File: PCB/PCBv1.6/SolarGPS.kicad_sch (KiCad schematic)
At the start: 44 parts, among them J1 Conn_01x10_Female, J2 Solar2+, J3 Solar1+, J4 GND, J5 GND, J6 Conn_02x03_Odd_Even, J7 Screw_Terminal_01x01, J8 Conn_01x04_Male, U1 BQ25505, U2 L96-M33, U3 STM32L031G6Ux, U4 MAX40200AUK, U6 LIS3DH, Y1 32.768

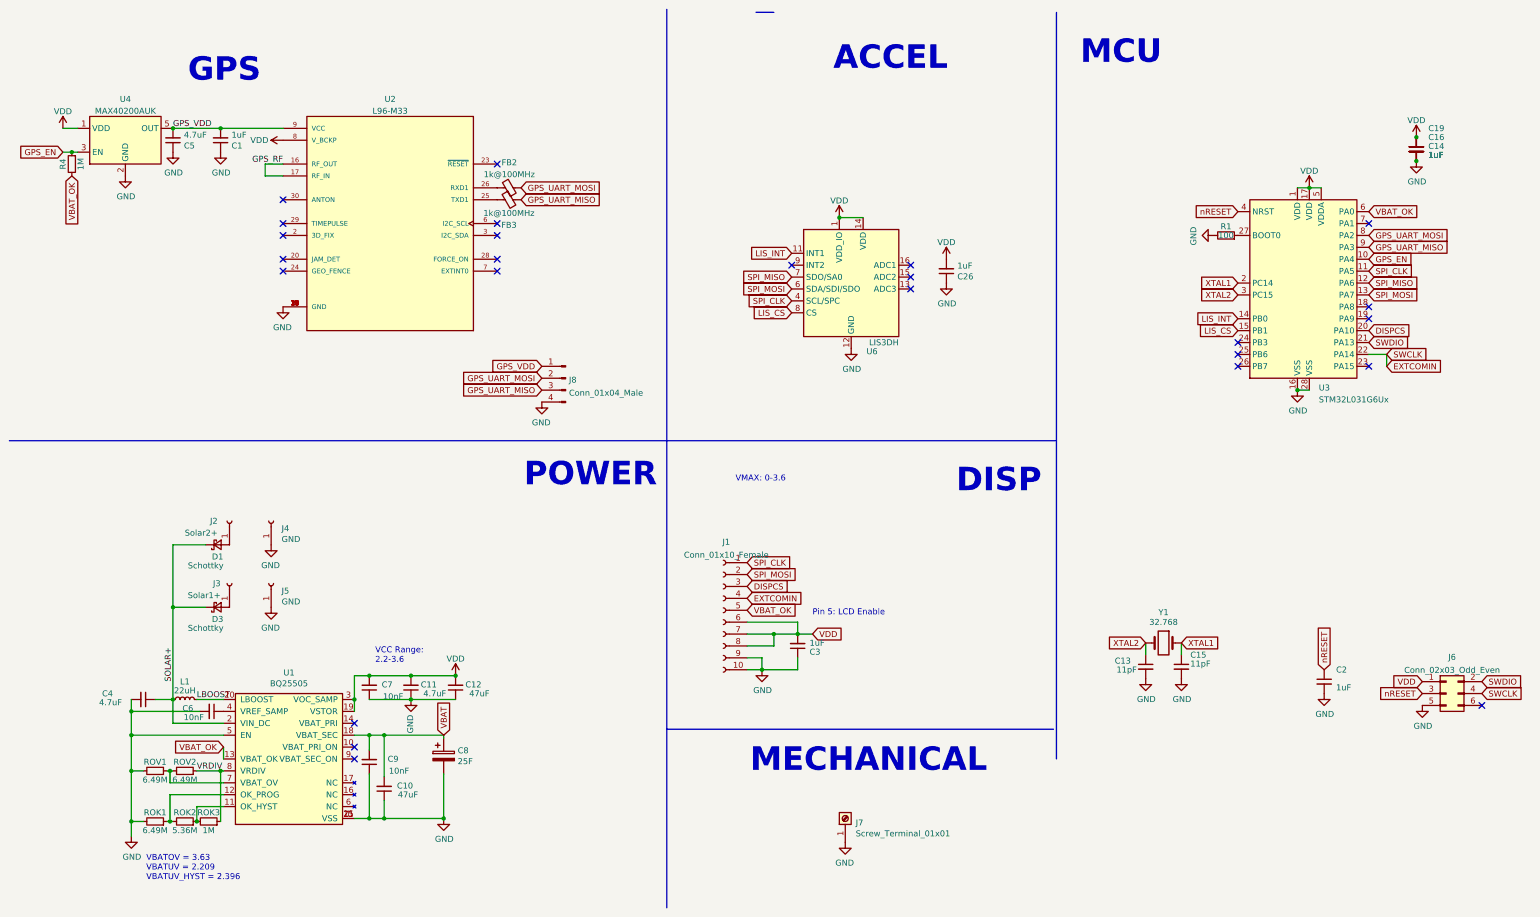
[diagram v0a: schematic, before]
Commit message: Update PCBV10
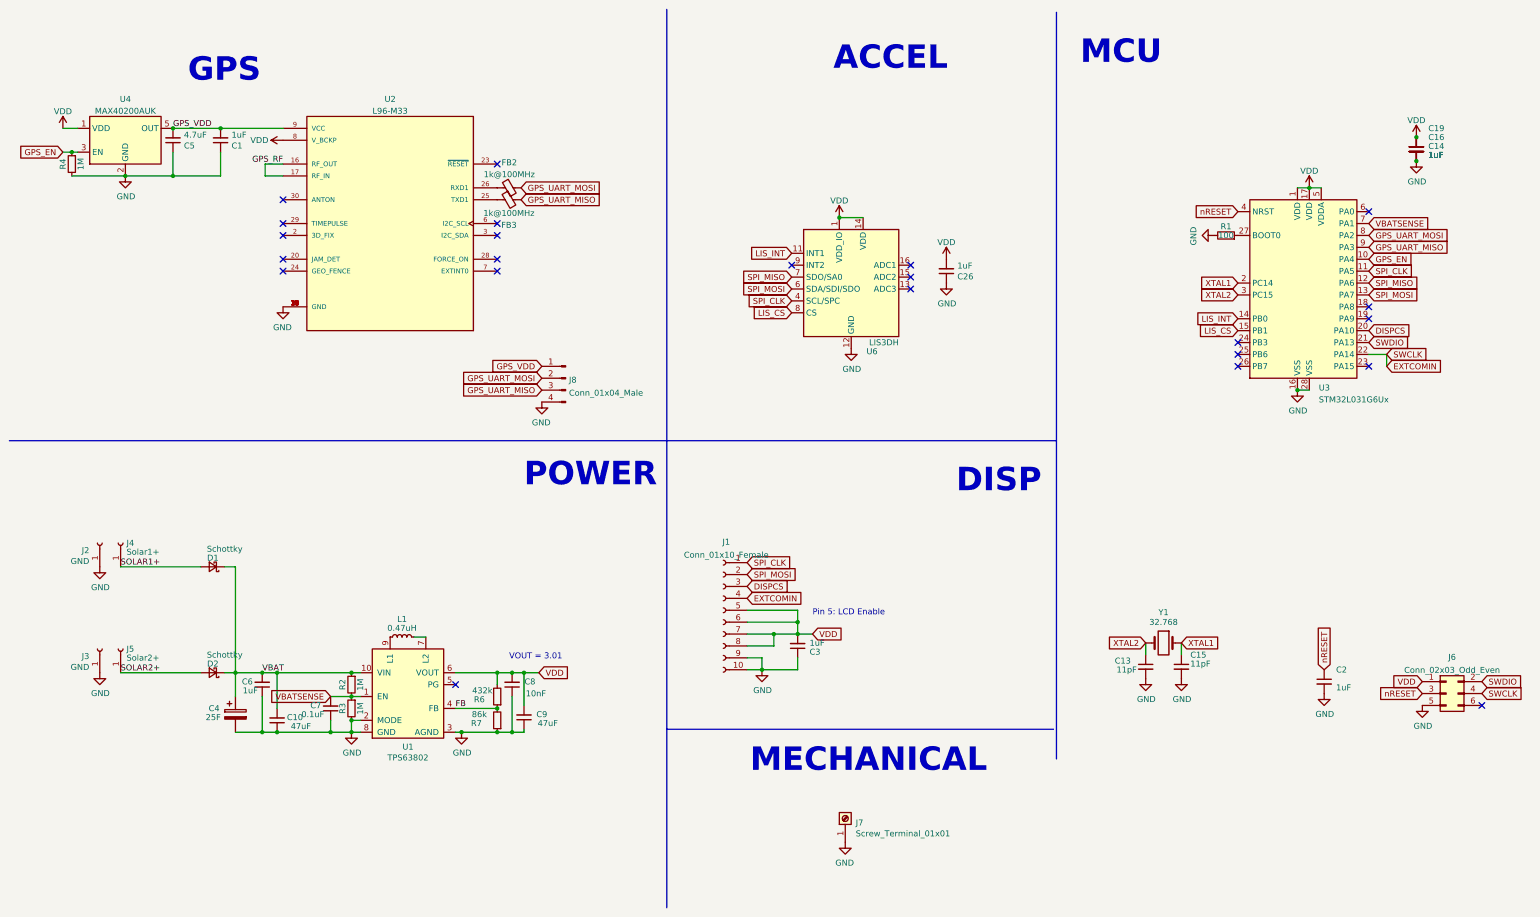
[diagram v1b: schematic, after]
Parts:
- removed C11, C4: 4.7uF, Capacitor_SMD:C_0805_2012Metric, symbol Device:C_Small
- removed C12: 47uF, Capacitor_SMD:C_1206_3216Metric, symbol Device:C_Small
- removed C8: 25F, Heliograph:TPLC3R8-25MR8X20, symbol Device:C_Polarized
- removed D3: Schottky, Diode_SMD:D_SOD-323_HandSoldering, symbol Device:D_Schottky_Small
- removed ROK1, ROV1, ROV2: 6.49M, Resistor_SMD:R_0603_1608Metric, symbol Device:R_Small
- removed ROK2: 5.36M, Resistor_SMD:R_0603_1608Metric, symbol Device:R_Small
- removed ROK3: 1M, Resistor_SMD:R_0603_1608Metric, symbol Device:R_Small
- removed U1: BQ25505, Package_DFN_QFN:Texas_VQFN-RGR-20, symbol MargoGeneral:BQ25505
- added C4: 25F, Heliograph:TPLC3R8-25MR8X20, symbol Device:C_Polarized
- added C8: 10nF, Capacitor_SMD:C_0603_1608Metric, symbol Device:C_Small
- added D2: Schottky, Diode_SMD:D_SOD-323_HandSoldering, symbol Device:D_Schottky_Small
- added R2, R3: 1M, Resistor_SMD:R_0603_1608Metric, symbol Device:R_Small
- added R6: 432k, Resistor_SMD:R_0603_1608Metric, symbol Device:R_Small
- added R7: 86k, Resistor_SMD:R_0603_1608Metric, symbol Device:R_Small
- added U1: TPS63802, Margo_Lib:VREG_TPS63802DLAR, symbol SolarGPS-rescue:TPS63802-VeridianDesigns
- C6: value 10nF -> 1uF
- C7: value 10nF -> 0.1uF
- C9: value 10nF -> 47uF; footprint Capacitor_SMD:C_0603_1608Metric -> Capacitor_SMD:C_1206_3216Metric
- J2: value Solar2+ -> GND
- J3: value Solar1+ -> GND
- J4: value GND -> Solar1+
- J5: value GND -> Solar2+
- L1: value 22uH -> 0.47uH; footprint Heliograph:744031220 -> Inductor_SMD:L_0805_2012Metric_Pad1.05x1.20mm_HandSolder; Part 744031220 -> DFE201612E
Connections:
- net GND: now also C6.1, J2.1 (Pin_1), J3.1 (Pin_1), R4.2, C4.2, C8.1, R3.2, R7.1, U1.2 (MODE), U1.3 (AGND), U1.8 (GND); no longer C6.2, J4.1 (Pin_1), J5.1 (Pin_1)
- net VBAT: now also C6.2, D1.1 (K), C4.1, D2.1 (K), R2.1, U1.10 (VIN); no longer C9.2
- net VDD: now also C9.2, J1.5 (Pin_5), C8.2, R6.2, U1.6 (VOUT); no longer C7.2
- net VBATSENSE: now reaches U3.7 (PA1)
- net VBATSENSE: now also C7.2, R2.2, R3.1, U1.1 (EN)
- net SOLAR1+: now reaches D1.2 (A)
- net SOLAR1+: now also J4.1 (Pin_1); no longer J2.1 (Pin_1)
- net LBOOST: no longer names the net of L1.2
- net LBOOST: now also U1.7 (L2)
- net SOLAR+: no longer names the net of L1.1
- net SOLAR+: now also U1.9 (L1); no longer D1.1 (K)
- removed net VBAT_OK: J1.5 (Pin_5), R4.2, U3.6 (PA0)
- new net FB: R6.1, R7.2, U1.4 (FB)
- new net SOLAR2+: D2.2 (A), J5.1 (Pin_1)
- no-connect marks 25 -> 23
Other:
- note added: "VOUT = 3.01"
- note removed: "VBATOV = 3.63 VBATUV = 2.209 VBATUV_HYST = 2.396"
- note removed: "VCC Range: 2.2-3.6"
- note removed: "VMAX: 0-3.6"

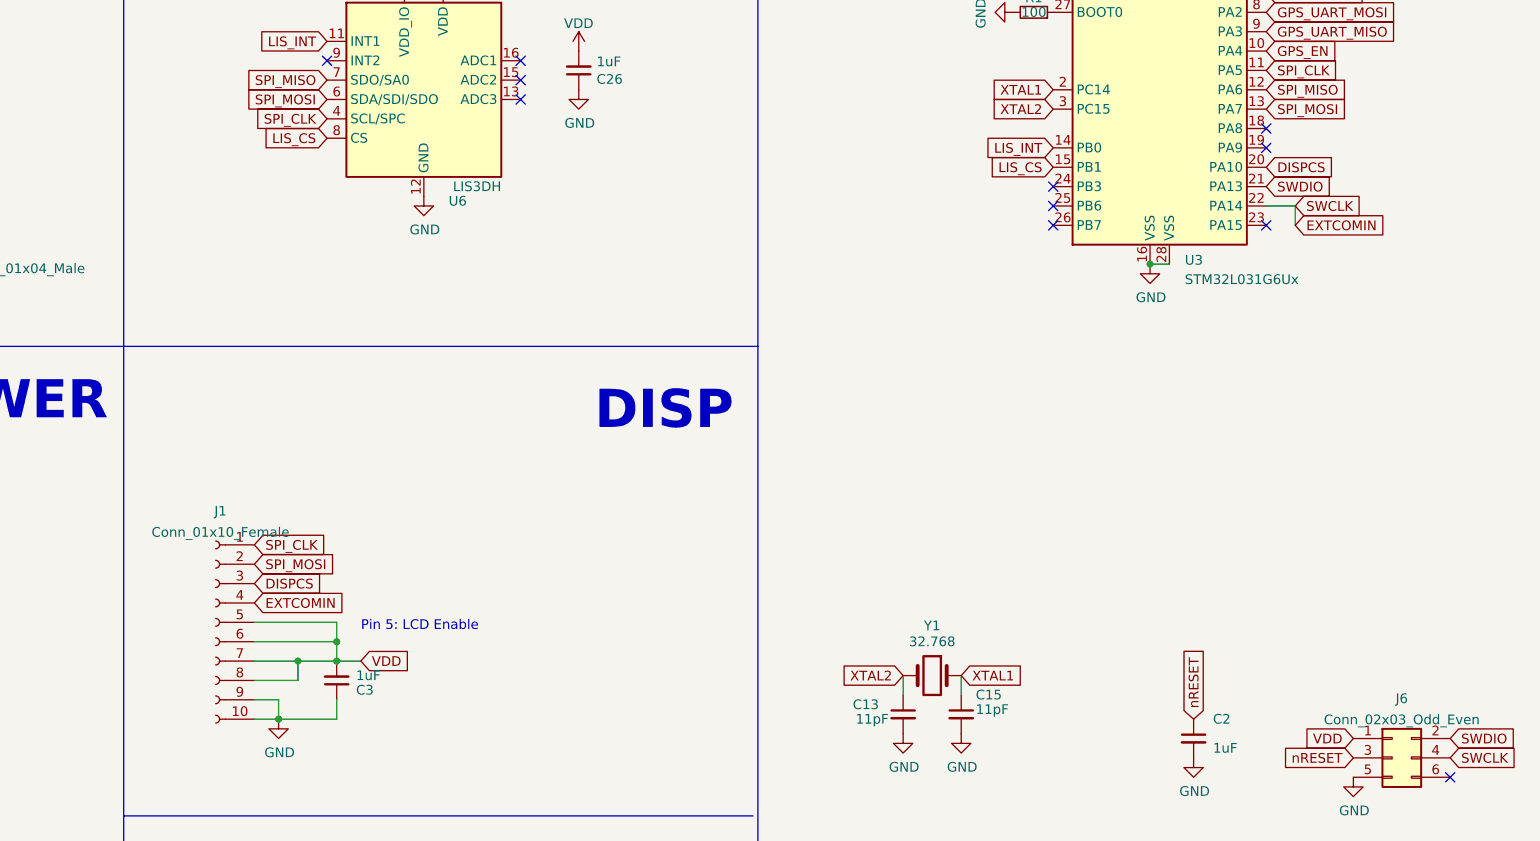
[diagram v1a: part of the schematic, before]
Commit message: PCB1.6
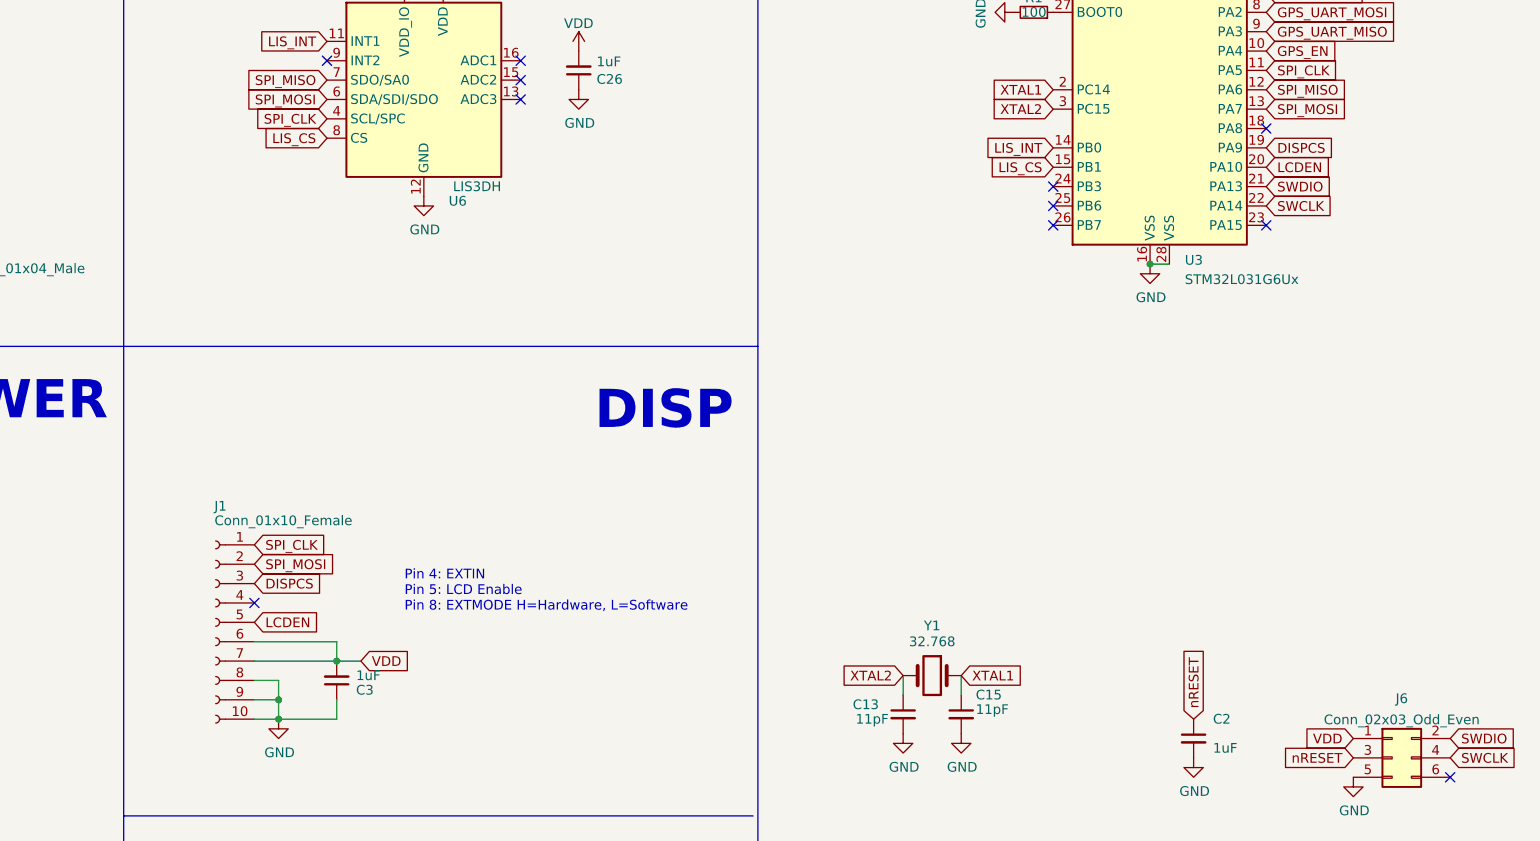
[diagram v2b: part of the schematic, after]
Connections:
- net DISPCS: now also U3.19 (PA9); no longer U3.20 (PA10)
- net GND: now also J1.8 (Pin_8)
- net VDD: no longer J1.5 (Pin_5), J1.8 (Pin_8)
- net EXTCOMIN renamed SWCLK
- net SWCLK: no longer J1.4 (Pin_4)
- new net LCDEN: J1.5 (Pin_5), U3.20 (PA10)
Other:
- note added: "Pin 4: EXTIN Pin 5: LCD Enable Pin 8: EXTMODE H=Hardware, L=Software"
- note removed: "Pin 5: LCD Enable"
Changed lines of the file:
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@@
   (junction (at 66.04 153.035) (diameter 0) (color 0 0 0 0)
   )
-  (junction (at 180.34 142.24) (diameter 0) (color 0 0 0 0)
-  )
   (junction (at 57.15 36.83) (diameter 0) (color 0 0 0 0)
   )
@@
   (junction (at 85.09 163.195) (diameter 0) (color 0 0 0 0)
   )
+  (junction (at 172.72 149.86) (diameter 0) (color 0 0 0 0)
+  )
   (junction (at 66.04 165.735) (diameter 0) (color 0 0 0 0)
   )
@@
   (junction (at 119.38 165.735) (diameter 0) (color 0 0 0 0)
   )
-  (junction (at 175.26 144.78) (diameter 0) (color 0 0 0 0)
-  )
   (junction (at 46.99 46.99) (diameter 0) (color 0 0 0 0)
   )
-  (no_connect (at 302.26 77.47))
+  (no_connect (at 169.545 137.16))
   (no_connect (at 204.47 71.12))
   (no_connect (at 107.315 155.575))
@@
     (stroke (width 0) (type default) (color 0 0 0 0))
   )
-  (wire (pts (xy 180.34 139.7) (xy 169.545 139.7))
-    (stroke (width 0) (type default) (color 0 0 0 0))
-  )
   (wire (pts (xy 172.72 149.86) (xy 172.72 152.4))
     (stroke (width 0) (type default) (color 0 0 0 0))
@@
     (stroke (width 0) (type default) (color 0 0 0 0))
   )
-  (wire (pts (xy 175.26 147.32) (xy 175.26 144.78))
+  (wire (pts (xy 172.72 149.86) (xy 172.72 147.32))
     (stroke (width 0) (type default) (color 0 0 0 0))
   )
@@
     (stroke (width 0) (type default) (color 0 0 0 0))
   )
+  (wire (pts (xy 172.72 147.32) (xy 169.545 147.32))
+    (stroke (width 0) (type default) (color 0 0 0 0))
+  )
   (polyline (pts (xy 12.065 103.505) (xy 235.585 103.505))
     (stroke (width 0) (type default) (color 0 0 0 0))
@@
     (stroke (width 0) (type default) (color 0 0 0 0))
   )
-  (wire (pts (xy 169.545 147.32) (xy 175.26 147.32))
-    (stroke (width 0) (type default) (color 0 0 0 0))
-  )
   (wire (pts (xy 85.09 163.195) (xy 86.995 163.195))
     (stroke (width 0) (type default) (color 0 0 0 0))
@@
     (stroke (width 0) (type default) (color 0 0 0 0))
   )
-  (wire (pts (xy 169.545 144.78) (xy 175.26 144.78))
+  (wire (pts (xy 169.545 144.78) (xy 180.34 144.78))
     (stroke (width 0) (type default) (color 0 0 0 0))
   )
@@
     (stroke (width 0) (type default) (color 0 0 0 0))
   )
-  (wire (pts (xy 180.34 142.24) (xy 180.34 139.7))
-    (stroke (width 0) (type default) (color 0 0 0 0))
-  )
   (wire (pts (xy 25.4 46.99) (xy 36.83 46.99))
     (stroke (width 0) (type default) (color 0 0 0 0))
   )
-  (wire (pts (xy 175.26 144.78) (xy 180.34 144.78))
-    (stroke (width 0) (type default) (color 0 0 0 0))
-  )
   (wire (pts (xy 85.09 163.195) (xy 85.09 165.735))
     (stroke (width 0) (type default) (color 0 0 0 0))
@@
     (stroke (width 0) (type default) (color 0 0 0 0))
   )
-  (wire (pts (xy 302.26 85.09) (xy 306.07 85.09))
-    (stroke (width 0) (type default) (color 0 0 0 0))
-  )
   (wire (pts (xy 36.83 46.99) (xy 46.99 46.99))
     (stroke (width 0) (type default) (color 0 0 0 0))
@@
   )
   (wire (pts (xy 107.315 153.035) (xy 116.205 153.035))
-    (stroke (width 0) (type default) (color 0 0 0 0))
-  )
-  (wire (pts (xy 306.07 87.63) (xy 306.07 85.09))
     (stroke (width 0) (type default) (color 0 0 0 0))
   )
@@
     (effects (font (size 5.0038 5.0038) (thickness 1.0008) bold) (justify left bottom))
   )
-  (text "Pin 5: LCD Enable" (at 183.515 140.97 0)
+  (text "Pin 4: EXTIN\nPin 5: LCD Enable\nPin 8: EXTMODE H=Hardware, L=Software"
+    (at 189.23 138.43 0)
     (effects (font (size 1.27 1.27)) (justify left bottom))
   )
@@
     )
   )
+  (global_label "LCDEN" (shape input) (at 302.26 80.01 0) (fields_autoplaced)
+    (effects (font (size 1.27 1.27)) (justify left))
+    (property "Intersheet References" "${INTERSHEET_REFS}" (id 0) (at 310.6318 79.9306 0)
+      (effects (font (size 1.27 1.27)) (justify left) hide)
+    )
+  )
   (global_label "GPS_UART_MISO" (shape input) (at 121.285 52.07 0) (fields_autoplaced)
     (effects (font (size 1.27 1.27)) (justify left))
@@
     )
   )
-  (global_label "DISPCS" (shape input) (at 302.26 80.01 0) (fields_autoplaced)
-    (effects (font (size 1.27 1.27)) (justify left))
-    (property "Intersheet References" "${INTERSHEET_REFS}" (id 0) (at 311.418 79.9306 0)
+  (global_label "DISPCS" (shape input) (at 302.26 77.47 0) (fields_autoplaced)
+    (effects (font (size 1.27 1.27)) (justify left))
+    (property "Intersheet References" "${INTERSHEET_REFS}" (id 0) (at 311.418 77.3906 0)
       (effects (font (size 1.27 1.27)) (justify left) hide)
     )
@@
     )
   )
-  (global_label "EXTCOMIN" (shape input) (at 306.07 87.63 0) (fields_autoplaced)
-    (effects (font (size 1.27 1.27)) (justify left))
-    (property "Intersheet References" "${INTERSHEET_REFS}" (id 0) (at 317.7075 87.5506 0)
-      (effects (font (size 1.27 1.27)) (justify left) hide)
-    )
-  )
   (global_label "SWDIO" (shape input) (at 302.26 82.55 0) (fields_autoplaced)
     (effects (font (size 1.27 1.27)) (justify left))
@@
     )
   )
-  (global_label "EXTCOMIN" (shape input) (at 169.545 137.16 0) (fields_autoplaced)
-    (effects (font (size 1.27 1.27)) (justify left))
-    (property "Intersheet References" "${INTERSHEET_REFS}" (id 0) (at 181.1825 137.0806 0)
-      (effects (font (size 1.27 1.27)) (justify left) hide)
-    )
-  )
   (global_label "SPI_MOSI" (shape input) (at 169.545 132.08 0) (fields_autoplaced)
     (effects (font (size 1.27 1.27)) (justify left))
@@
     )
   )
-  (global_label "SWCLK" (shape input) (at 306.07 85.09 0) (fields_autoplaced)
-    (effects (font (size 1.27 1.27)) (justify left))
-    (property "Intersheet References" "${INTERSHEET_REFS}" (id 0) (at 314.6232 85.0106 0)
+  (global_label "SWCLK" (shape input) (at 302.26 85.09 0) (fields_autoplaced)
+    (effects (font (size 1.27 1.27)) (justify left))
+    (property "Intersheet References" "${INTERSHEET_REFS}" (id 0) (at 310.8132 85.0106 0)
       (effects (font (size 1.27 1.27)) (justify left) hide)
     )
@@
     (property "Intersheet References" "${INTERSHEET_REFS}" (id 0) (at 246.8075 146.6056 0)
       (effects (font (size 1.27 1.27)) (justify right) hide)
+    )
+  )
+  (global_label "LCDEN" (shape input) (at 169.545 139.7 0) (fields_autoplaced)
+    (effects (font (size 1.27 1.27)) (justify left))
+    (property "Intersheet References" "${INTERSHEET_REFS}" (id 0) (at 177.9168 139.6206 0)
+      (effects (font (size 1.27 1.27)) (justify left) hide)
     )
   )
@@
   )
   (symbol (lib_id "Connector:Conn_01x10_Female") (at 164.465 139.7 0) (mirror y) (unit 1)
-    (in_bom yes) (on_board yes) (fields_autoplaced)
-    (property "Reference" "J1" (id 0) (at 165.1 125.1163 0))
-    (property "Value" "Conn_01x10_Female" (id 1) (at 165.1 127.8914 0))
+    (in_bom yes) (on_board yes)
+    (property "Reference" "J1" (id 0) (at 165.1 124.46 0))
+    (property "Value" "Conn_01x10_Female" (id 1) (at 173.355 126.365 0))
     (property "Footprint" "Heliograph:LS013B7DH03" (id 2) (at 164.465 139.7 0)
       (effects (font (size 1.27 1.27)) hide)
